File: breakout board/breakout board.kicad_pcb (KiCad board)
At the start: 2 copper layers, 3 parts, among them J1 Conn_01x07_Pin, J2 Conn_01x07_Pin, U1 MCP2518FD-xQBB

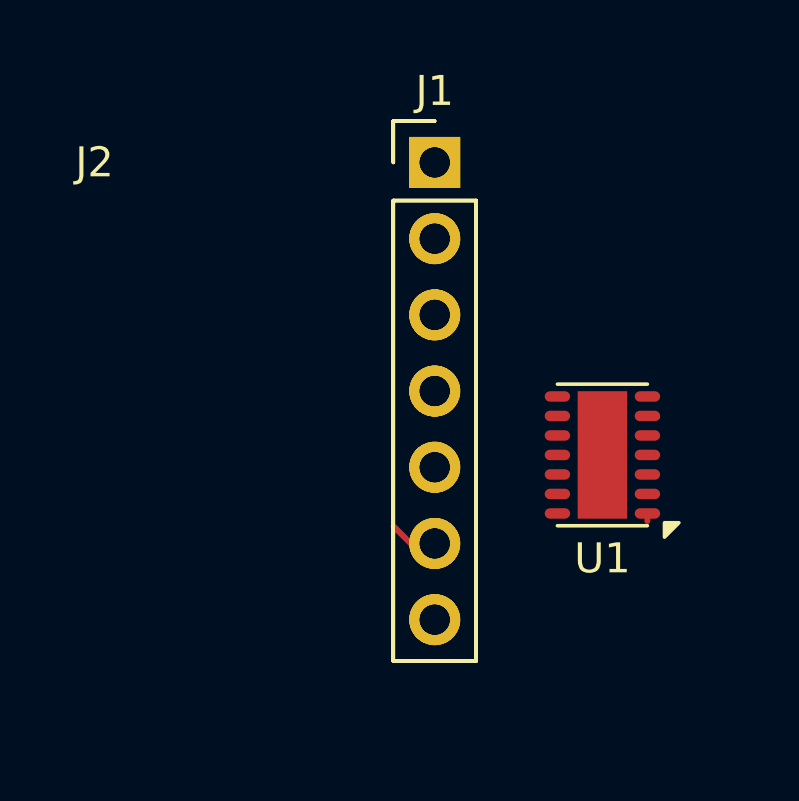
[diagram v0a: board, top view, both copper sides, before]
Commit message: work
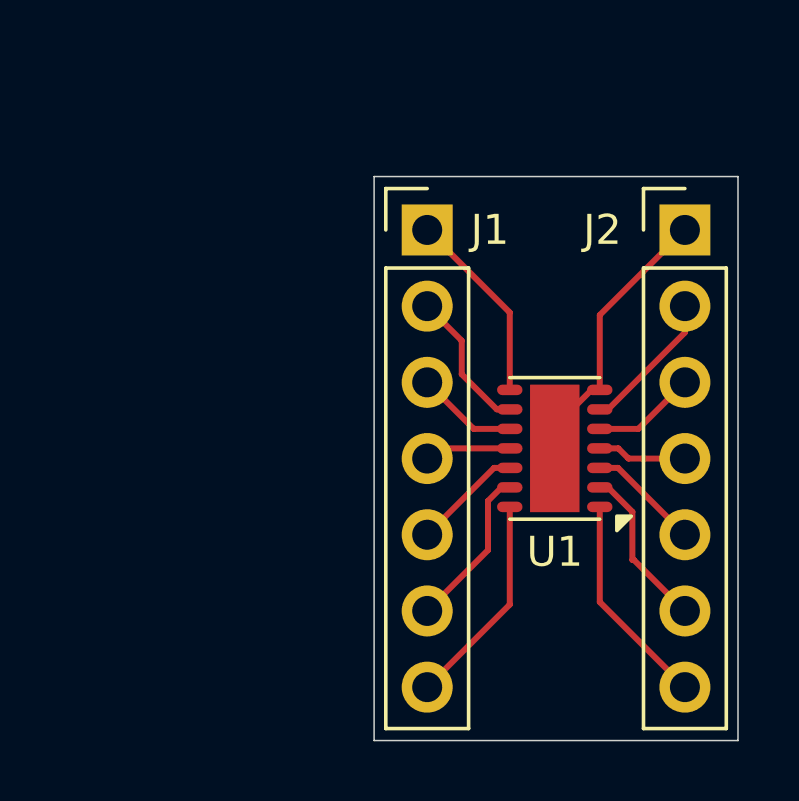
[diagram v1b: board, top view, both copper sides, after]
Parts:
- moved J2 8.64 mm to (130.5, 96.5)
- moved J1 2.26 mm to (121.9, 96.5)
- moved U1 1.60 mm to (126.2, 103.8)
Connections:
- U1 pad 1: Net-(J2-Pin_5) -> Net-(J2-Pin_7)
- U1 pad 10: Net-(J1-Pin_4) -> Net-(J1-Pin_3)
- U1 pad 11: Net-(J1-Pin_1) -> Net-(J1-Pin_4)
- U1 pad 12: Net-(J1-Pin_2) -> Net-(J1-Pin_5)
- U1 pad 13: Net-(J1-Pin_3) -> Net-(J1-Pin_6)
- U1 pad 14: Net-(J2-Pin_7) -> Net-(J1-Pin_7)
- U1 pad 15: Net-(J1-Pin_7) -> Net-(J2-Pin_1)
- U1 pad 3: Net-(J2-Pin_4) -> Net-(J2-Pin_5)
- U1 pad 4: Net-(J2-Pin_3) -> Net-(J2-Pin_4)
- U1 pad 5: Net-(J1-Pin_5) -> Net-(J2-Pin_3)
- U1 pad 6: Net-(J1-Pin_6) -> Net-(J2-Pin_2)
- U1 pad 7: Net-(J1-Pin_7) -> Net-(J2-Pin_1)
- U1 pad 8: Net-(J2-Pin_1) -> Net-(J1-Pin_1)
- U1 pad 9: Net-(J2-Pin_2) -> Net-(J1-Pin_2)
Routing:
- net Net-(J2-Pin_1): track 0.00 -> 9.24 mm
- net Net-(J2-Pin_7): track 0.00 -> 7.18 mm
- net Net-(J1-Pin_7): track 0.00 -> 7.15 mm
- net Net-(J1-Pin_1): track 0.00 -> 6.47 mm
- net Net-(J2-Pin_6): track 0.28 -> 5.48 mm
- net Net-(J1-Pin_2): track 0.00 -> 4.83 mm
- net Net-(J2-Pin_2): track 0.00 -> 4.78 mm
- net Net-(J2-Pin_5): track 0.25 -> 3.76 mm
- net Net-(J1-Pin_6): track 1.92 -> 5.42 mm
- net Net-(J2-Pin_3): track 0.00 -> 3.48 mm
- net Net-(J1-Pin_5): track 0.27 -> 3.68 mm
- net Net-(J1-Pin_3): track 0.00 -> 3.40 mm
- net Net-(J2-Pin_4): track 0.00 -> 2.98 mm
- net Net-(J1-Pin_4): track 0.00 -> 2.89 mm
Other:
- board outline added: 12.1 x 18.8 mm
